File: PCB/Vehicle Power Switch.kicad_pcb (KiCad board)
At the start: 2 copper layers, 76.5 x 85 mm, 47 parts, among them J6 STX-3790-5N, J7 Debug Hdr, J8 AVR-UPDI-6, Q1 MMBT2222A, Q2 MMBT2222A, Q3 BSS84, U1 MCP1703Ax-250xxTT, U2 LIS2HH12, U3 ATtiny404-SS

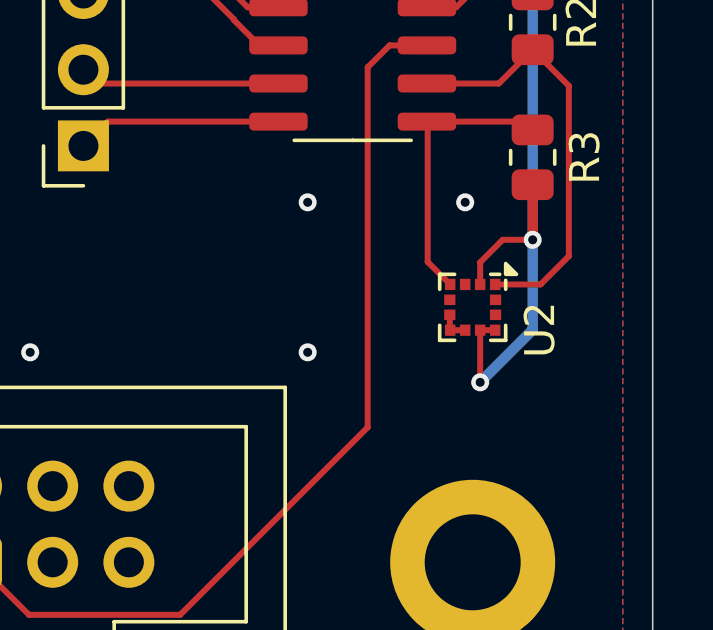
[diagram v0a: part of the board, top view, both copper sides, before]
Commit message: Fixes to PCB v2 and working on firmware.
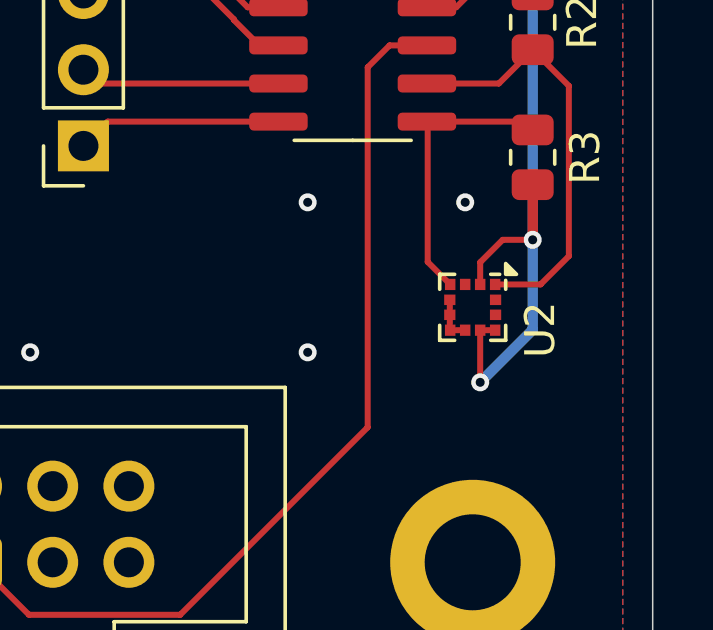
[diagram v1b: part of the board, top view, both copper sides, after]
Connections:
- U2 pad 5: unconnected-(U2-RES-Pad5) -> GND

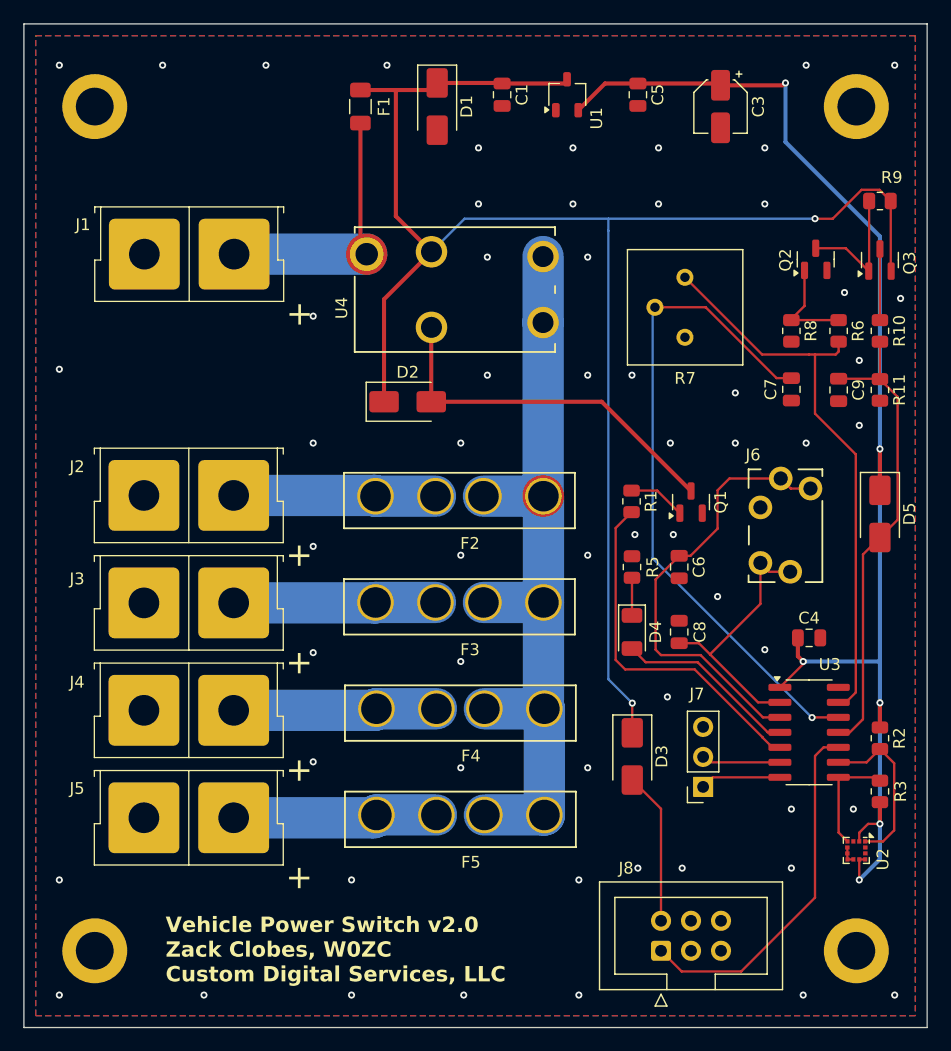
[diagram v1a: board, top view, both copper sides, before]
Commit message: All functionality is working on the prototype. Firmware is still rough.
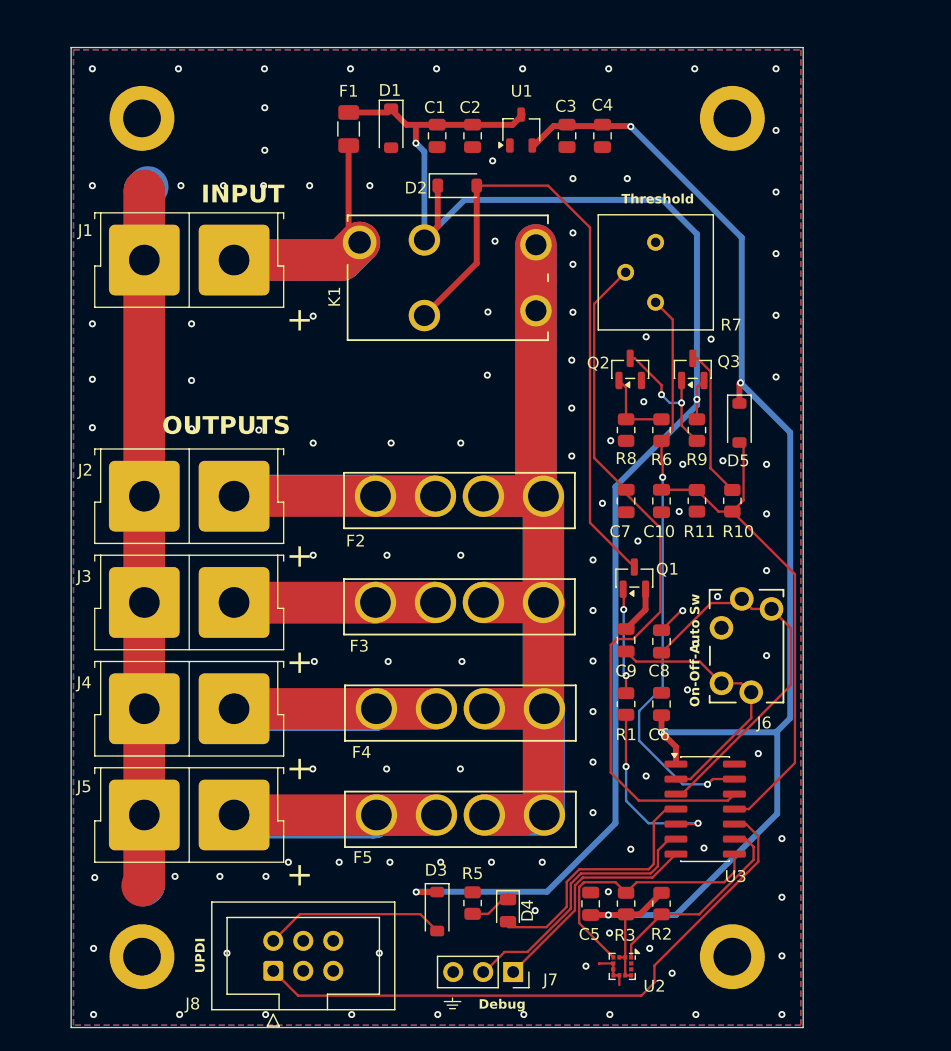
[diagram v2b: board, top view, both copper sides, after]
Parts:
- added C2: 10nF, Capacitor_SMD:C_0805_2012Metric, F.Cu at (94.0, 59.5)
- added C3: 22uF, Capacitor_SMD:C_0805_2012Metric, F.Cu at (102.0, 59.5)
- C1: value .1uF -> 22uF
- C10: renamed from C9; value .1uF -> 10nF
- C4: renamed from C3; value 10uF -> 10nF; footprint Capacitor_SMD:CP_Elec_4x5.3 -> Capacitor_SMD:C_0805_2012Metric
- C5: renamed from C4; value .1uF -> 10nF
- C6: renamed from C5; value .1uF -> 10nF
- C7: value .1uF -> 10nF
- C8: renamed from C6; value .1uF -> 10nF
- C9: renamed from C8; value .1uF -> 10nF
- D1, D2, D3, D5: value MRA4007T3G -> 1N4007FL; footprint Diode_SMD:D_SMA -> Diode_SMD:D_SOD-123
- D4: footprint LED_SMD:LED_1206_3216Metric -> LED_SMD:LED_0805_2012Metric
- moved C6 51.6 mm to (110.0, 107.6), turned to 90 degrees
- moved J8 32.9 mm to (77.1, 130.2)
- moved R5 31.5 mm to (94.0, 124.5)
- moved C5 29.1 mm to (104.0, 124.5), turned to 90 degrees
- moved D4 25.8 mm to (97.0, 125.1)
- moved R9 24.8 mm to (113.0, 84.4), turned to -90 degrees
- moved R3 23.5 mm to (107.0, 124.5)
- moved R2 23.2 mm to (110.0, 124.5)
- moved J7 22.5 mm to (97.4, 130.3), turned to -90 degrees
- moved U2 22.1 mm to (106.7, 129.8)
- moved D3 21.1 mm to (91.0, 125.2)
- moved R10 19.1 mm to (116.0, 90.4)
- moved D2 18.8 mm to (92.7, 63.7)
- moved Q3 18.4 mm to (112.7, 79.3)
- moved Q2 18.3 mm to (107.3, 79.3)
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- renumbered U4 to K1
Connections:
- R7 pad 1: Net-(U3-PA3) -> GND
- R7 pad 3: GND -> Net-(U3-PA3)
- U2 pad 3: unconnected-(U2-SA0/SDO-Pad3) -> +3V3
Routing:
- net GND: track 1.50 -> 128.4 mm, vias 59 -> 112
- net /1: track 69.4 -> 137.8 mm
- net /2: track 66.8 -> 129.6 mm
- net Net-(D2-A): track 31.8 -> 54.2 mm
- net Net-(J8-DATA): track 30.6 -> 52.1 mm
- net Net-(J7-Pin_2): track 6.69 -> 23.4 mm
- net Net-(U3-PA7): track 30.1 -> 16.1 mm, vias 0 -> 2
- net /PB1: track 9.89 -> 23.1 mm
- net Net-(J7-Pin_1): track 6.84 -> 19.2 mm
- net /In: track 22.6 -> 31.1 mm
- net Net-(Q3-D): track 6.03 -> 12.8 mm
- net Net-(D4-A): track 15.5 -> 21.7 mm
- net Net-(U3-PA5): track 37.8 -> 32.2 mm
- net +3V3: track 114.9 -> 120.3 mm, vias 6 -> 4
- net +BATT: track 139.1 -> 134.0 mm, vias 2 -> 3
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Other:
- board size 76.5 x 85 mm -> 62 x 83 mm
- board text added: "Debug"
- board text added: "INPUT"
- board text added: "OUTPUTS"
- board text added: "On-Off-Auto Sw"
- board text added: "Threshold"
- board text added: "UPDI"
- board text added: "Vehicle Power Switch v2.1.1 Zack Clobes, W0ZC Custom Digital Services, LLC"
- board text removed: "Vehicle Power Switch v2.0 Zack Clobes, W0ZC Custom Digital Services, LLC"
